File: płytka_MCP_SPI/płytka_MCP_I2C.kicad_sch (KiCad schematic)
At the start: 33 parts, among them J1 A0, J10 V0, J11 Ext, J12 I2C, J13 U2, J15 U2, J16 U3, J17 RS, J18 K, J19 A, J2 A1, J20 VDD, J21 GND, J23 VSS, J24 Conn_01x16_Pin, J25 LCD, J26 VCC, J3 A2, J4 SDA, J5 SCL, J6 INTA, J7 INTB, J8 INTA, J9 RESET, U1 MCP23017_SP

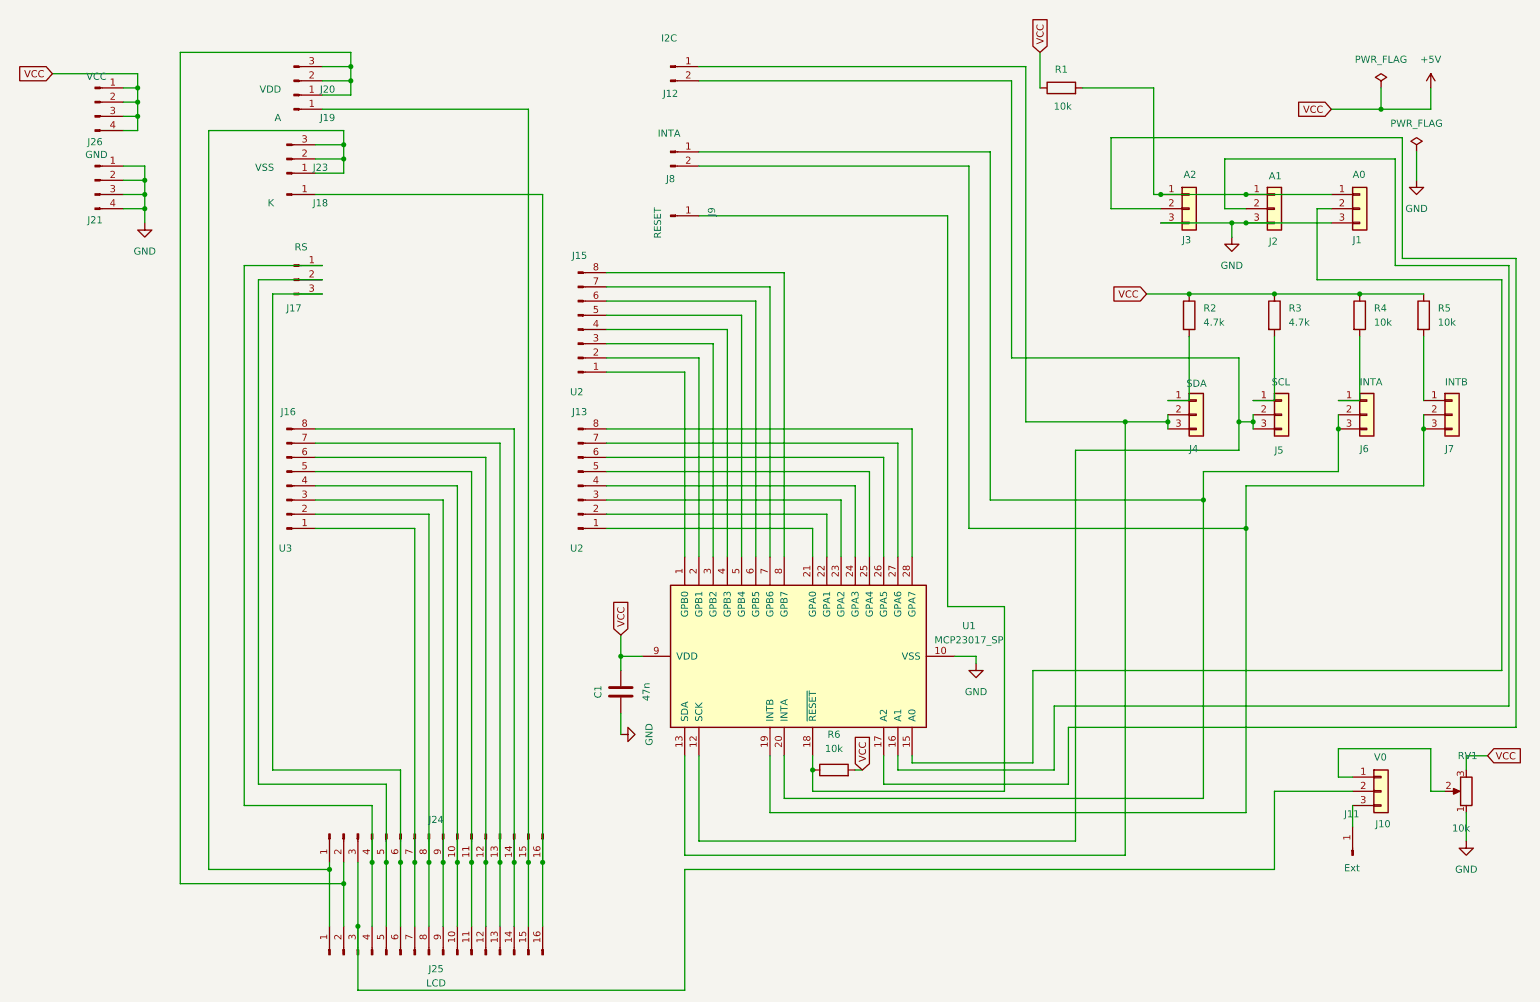
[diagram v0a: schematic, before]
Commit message: MCP_SPI płytka wersja 1.0
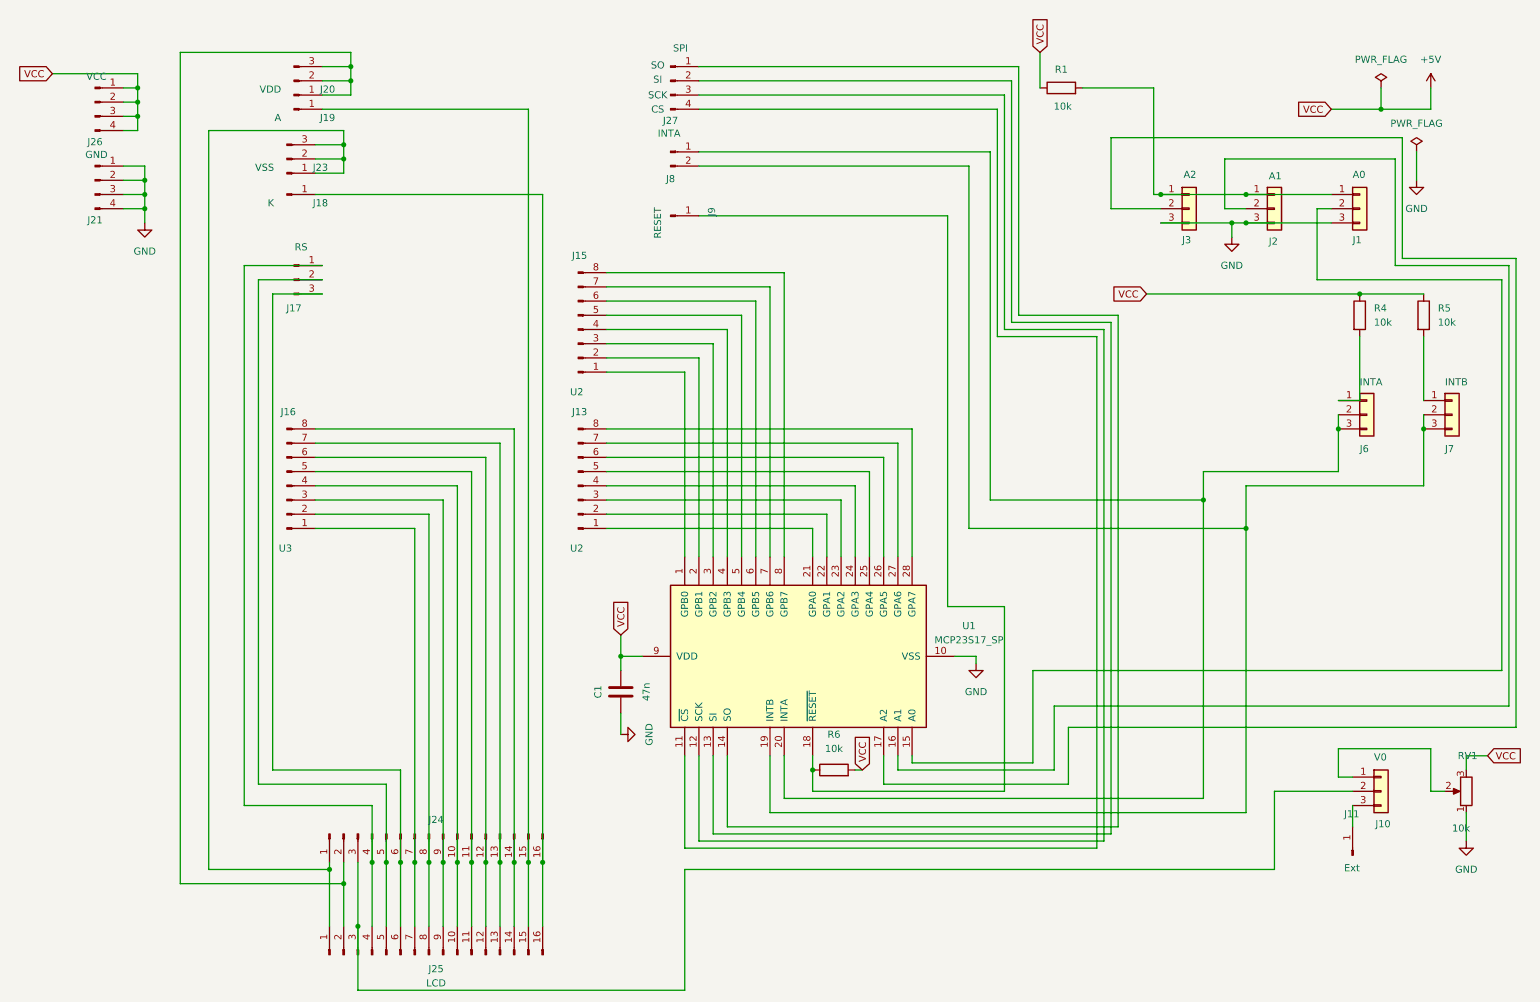
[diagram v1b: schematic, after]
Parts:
- removed J12: I2C, Connector_PinSocket_2.54mm:PinSocket_1x02_P2.54mm_Vertical, symbol Connector:Conn_01x02_Pin
- removed J4: SDA, Library:PinSocket_1x03_P2.54mm_Vertical, symbol Connector_Generic:Conn_01x03
- removed J5: SCL, Library:PinSocket_1x03_P2.54mm_Vertical, symbol Connector_Generic:Conn_01x03
- removed R2, R3: 4.7k, Library:R_Axial_DIN0207_L6.3mm_D2.5mm_P10.16mm_Horizontal_square, symbol Device:R
- removed U1: MCP23017_SP, Library:DIP-28_W7.62mm_LongPads_Edit, symbol Interface_Expansion:MCP23017_SP
- added J27: SPI, Connector_PinSocket_2.54mm:PinSocket_1x04_P2.54mm_Vertical, symbol Connector:Conn_01x04_Pin
- added U1: MCP23S17_SP, Library:DIP-28_W7.62mm_LongPads_Edit, symbol Interface_Expansion:MCP23S17_SP
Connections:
- net +5V: now also U1.9 (VDD)
- net GND: now also U1.10 (VSS)
- net at J15.1 (Pin_1): now also U1.1 (GPB0)
- net at J15.2 (Pin_2): now also U1.2 (GPB1)
- net at J15.3 (Pin_3): now also U1.3 (GPB2)
- net at J15.4 (Pin_4): now also U1.4 (GPB3)
- net at J15.5 (Pin_5): now also U1.5 (GPB4)
- net at J15.6 (Pin_6): now also U1.6 (GPB5)
- net at J15.7 (Pin_7): now also U1.7 (GPB6)
- net at J15.8 (Pin_8): now also U1.8 (GPB7)
- net at J3.2 (Pin_2): now also U1.17 (A2)
- net at J1.2 (Pin_2): now also U1.15 (A0)
- net at J6.2 (Pin_2), J6.3 (Pin_3), J8.1 (Pin_1): now also U1.20 (INTA)
- net at J7.2 (Pin_2), J7.3 (Pin_3), J8.2 (Pin_2): now also U1.19 (INTB)
- net at J2.2 (Pin_2): now also U1.16 (A1)
- net at J9.1 (Pin_1), R6.1: now also U1.18 (~{RESET})
- net at J13.1 (Pin_1): now also U1.21 (GPA0)
- net at J13.2 (Pin_2): now also U1.22 (GPA1)
- net at J13.3 (Pin_3): now also U1.23 (GPA2)
- net at J13.4 (Pin_4): now also U1.24 (GPA3)
- net at J13.5 (Pin_5): now also U1.25 (GPA4)
- net at J13.6 (Pin_6): now also U1.26 (GPA5)
- net at J13.7 (Pin_7): now also U1.27 (GPA6)
- net at J13.8 (Pin_8): now also U1.28 (GPA7)
- new net: J27.4 (Pin_4), U1.11 (~{CS})
- new net: J27.3 (Pin_3), U1.12 (SCK)
- new net: J27.2 (Pin_2), U1.13 (SI)
- new net: J27.1 (Pin_1), U1.14 (SO)
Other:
- note added: "CS"
- note added: "SCK"
- note added: "SI"
- note added: "SO"
- note added: "SPI"
